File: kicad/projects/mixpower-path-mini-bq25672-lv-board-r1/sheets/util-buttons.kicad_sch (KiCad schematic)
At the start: 15 parts, among them SW1 TS-A002, SW2 TS-A002, SW3 TS-A002, U11 RT9829GQW, U9 RT9829GQW

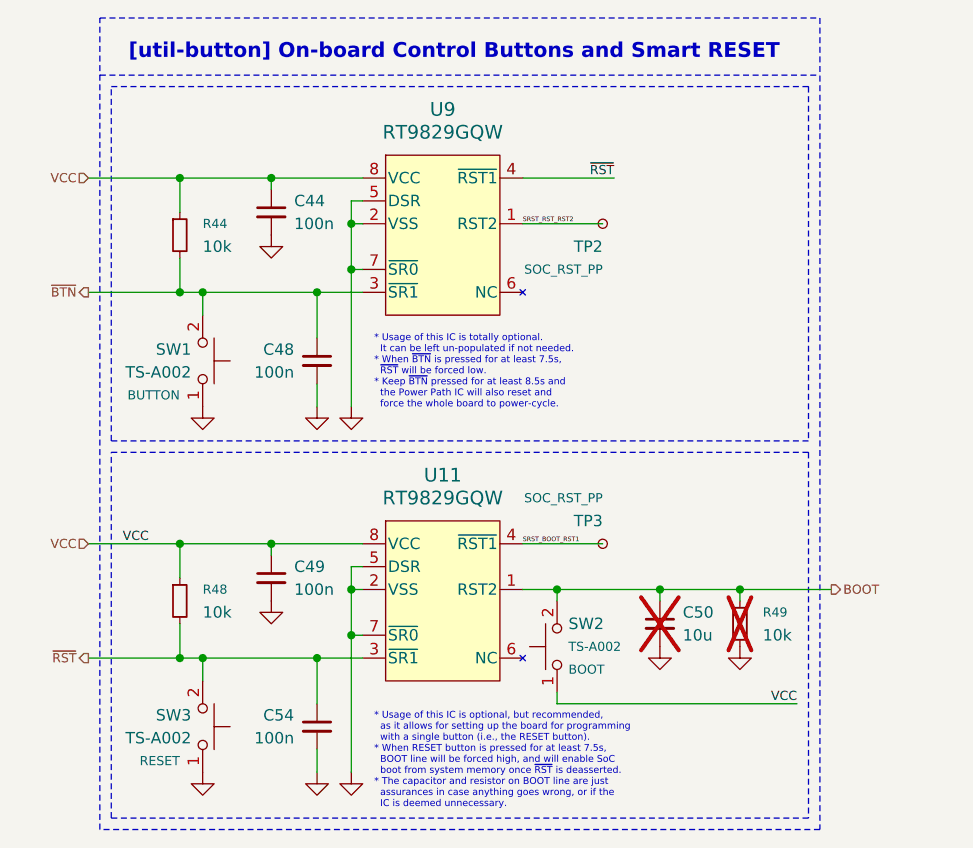
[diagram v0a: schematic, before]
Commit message: feat: small changes in schematics, some PCB routing
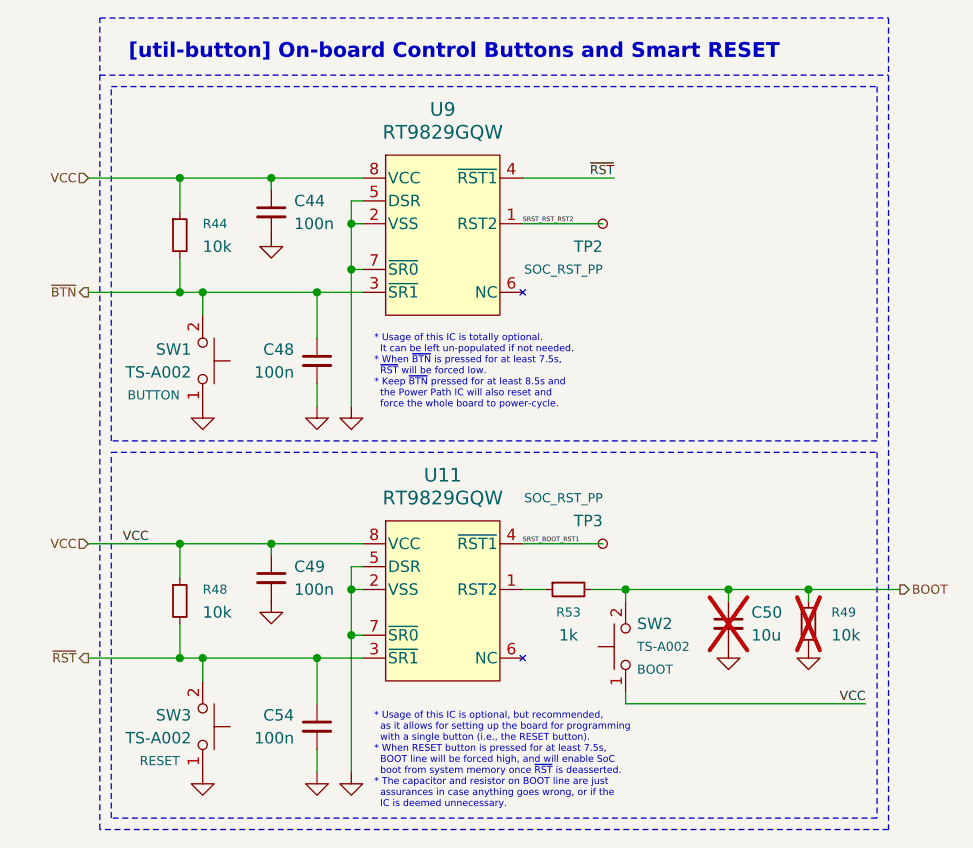
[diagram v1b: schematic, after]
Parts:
- added R53: 1k, Resistor_SMD:R_0402_1005Metric, symbol Device:R_Small
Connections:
- net BOOT: now also R53.2; no longer U11.1 (RST2)
- new net: R53.1, U11.1 (RST2)
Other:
- moved on the sheet: C50, R49, SW2
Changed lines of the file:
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@@
 	(rectangle
 		(start 68.58 24.13)
-		(end 146.05 63.5)
+		(end 153.67 63.5)
 		(stroke
 			(width 0)
@@
 	(rectangle
 		(start 67.31 16.51)
-		(end 147.32 106.68)
+		(end 154.94 106.68)
 		(stroke
 			(width 0)
@@
 	(rectangle
 		(start 68.58 64.77)
-		(end 146.05 105.41)
+		(end 153.67 105.41)
 		(stroke
 			(width 0)
@@
 	)
 	(junction
-		(at 129.54 80.01)
+		(at 137.16 80.01)
 		(diameter 0)
 		(color 0 0 0 0)
@@
 	)
 	(junction
-		(at 138.43 80.01)
+		(at 146.05 80.01)
 		(diameter 0)
 		(color 0 0 0 0)
@@
 	)
 	(junction
-		(at 118.11 80.01)
+		(at 125.73 80.01)
 		(diameter 0)
 		(color 0 0 0 0)
@@
 	(wire
 		(pts
-			(xy 129.54 80.01) (xy 138.43 80.01)
+			(xy 137.16 80.01) (xy 146.05 80.01)
 		)
 		(stroke
@@
 	(wire
 		(pts
-			(xy 118.11 80.01) (xy 118.11 81.28)
+			(xy 125.73 80.01) (xy 125.73 81.28)
 		)
 		(stroke
@@
 	(wire
 		(pts
+			(xy 121.92 80.01) (xy 125.73 80.01)
+		)
+		(stroke
+			(width 0)
+			(type default)
+		)
+	)
+	(wire
+		(pts
 			(xy 95.25 77.47) (xy 95.25 80.01)
 		)
@@
 	(polyline
 		(pts
-			(xy 67.31 22.86) (xy 147.32 22.86)
+			(xy 67.31 22.86) (xy 154.94 22.86)
 		)
 		(stroke
@@
 	(wire
 		(pts
-			(xy 129.54 80.01) (xy 129.54 81.28)
+			(xy 137.16 80.01) (xy 137.16 81.28)
 		)
 		(stroke
@@
 	(wire
 		(pts
-			(xy 118.11 92.71) (xy 144.78 92.71)
+			(xy 125.73 92.71) (xy 152.4 92.71)
 		)
 		(stroke
@@
 	(wire
 		(pts
-			(xy 114.3 80.01) (xy 118.11 80.01)
+			(xy 114.3 80.01) (xy 116.84 80.01)
 		)
 		(stroke
@@
 	(wire
 		(pts
-			(xy 138.43 80.01) (xy 148.59 80.01)
+			(xy 146.05 80.01) (xy 156.21 80.01)
 		)
 		(stroke
@@
 	(wire
 		(pts
-			(xy 118.11 91.44) (xy 118.11 92.71)
+			(xy 125.73 91.44) (xy 125.73 92.71)
 		)
 		(stroke
@@
 	(wire
 		(pts
-			(xy 138.43 80.01) (xy 138.43 81.28)
+			(xy 146.05 80.01) (xy 146.05 81.28)
 		)
 		(stroke
@@
 	(wire
 		(pts
-			(xy 118.11 80.01) (xy 129.54 80.01)
+			(xy 125.73 80.01) (xy 137.16 80.01)
 		)
 		(stroke
@@
 	)
 	(label "VCC"
-		(at 144.78 92.71 180)
+		(at 152.4 92.71 180)
 		(effects
 			(font
@@
 	(hierarchical_label "BOOT"
 		(shape output)
-		(at 148.59 80.01 0)
+		(at 156.21 80.01 0)
 		(effects
 			(font
@@
 	(symbol
 		(lib_id "mixlib-electromechanic-switch:TS-A002")
-		(at 118.11 86.36 90)
+		(at 125.73 86.36 90)
 		(unit 1)
 		(exclude_from_sim no)
@@
 		(dnp no)
 		(property "Reference" "SW2"
-			(at 119.38 83.8199 90)
+			(at 127 83.8199 90)
 			(effects
 				(font
@@
 		)
 		(property "Value" "TS-A002"
-			(at 119.38 86.3599 90)
+			(at 127 86.3599 90)
 			(effects
 				(font
@@
 		)
 		(property "Footprint" "mixlib-electromechanic-switch:TS-A002"
-			(at 118.11 86.36 0)
+			(at 125.73 86.36 0)
 			(effects
 				(font
@@
 		)
 		(property "Datasheet" "https://www.hq-dz.com/uploadfile/2024/0305/20240305025619371.pdf"
-			(at 123.444 85.852 0)
+			(at 131.064 85.852 0)
 			(effects
 				(font
@@
 		)
 		(property "Description" "12V 50mA 0.1Ohm MINIATURE SMD SPST BUTTON"
-			(at 124.206 86.868 0)
+			(at 131.826 86.868 0)
 			(effects
 				(font
@@
 		)
 		(property "Role" "BOOT"
-			(at 119.38 88.9 90)
+			(at 127 88.9 90)
 			(effects
 				(font
@@
 	(symbol
 		(lib_id "Device:C_Small")
-		(at 129.54 83.82 0)
+		(at 137.16 83.82 0)
 		(unit 1)
 		(exclude_from_sim no)
@@
 		(dnp yes)
 		(property "Reference" "C50"
-			(at 132.08 82.5562 0)
+			(at 139.7 82.5562 0)
 			(effects
 				(font
@@
 		)
 		(property "Value" "10u"
-			(at 132.08 85.0962 0)
+			(at 139.7 85.0962 0)
 			(effects
 				(font
@@
 		)
 		(property "Footprint" "Capacitor_SMD:C_0402_1005Metric"
-			(at 129.54 83.82 0)
+			(at 137.16 83.82 0)
 			(effects
 				(font
@@
 		)
 		(property "Datasheet" "~"
-			(at 129.54 83.82 0)
+			(at 137.16 83.82 0)
 			(effects
 				(font
@@
 		)
 		(property "Description" "Unpolarized capacitor, small symbol"
-			(at 129.54 83.82 0)
+			(at 137.16 83.82 0)
 			(effects
 				(font
@@
 	(symbol
 		(lib_id "power:GND")
-		(at 129.54 86.36 0)
+		(at 137.16 86.36 0)
 		(unit 1)
 		(exclude_from_sim no)
@@
 		(fields_autoplaced yes)
 		(property "Reference" "#PWR082"
-			(at 129.54 92.71 0)
+			(at 137.16 92.71 0)
 			(effects
 				(font
@@
 		)
 		(property "Value" "GND"
-			(at 129.54 91.44 0)
+			(at 137.16 91.44 0)
 			(effects
 				(font
@@
 		)
 		(property "Footprint" ""
-			(at 129.54 86.36 0)
+			(at 137.16 86.36 0)
 			(effects
 				(font
@@
 		)
 		(property "Datasheet" ""
-			(at 129.54 86.36 0)
+			(at 137.16 86.36 0)
 			(effects
 				(font
@@
 		)
 		(property "Description" "Power symbol creates a global label with name \"GND\" , ground"
-			(at 129.54 86.36 0)
+			(at 137.16 86.36 0)
 			(effects
 				(font
@@
 	(symbol
 		(lib_id "power:GND")
-		(at 138.43 86.36 0)
+		(at 146.05 86.36 0)
 		(unit 1)
 		(exclude_from_sim no)
@@
 		(fields_autoplaced yes)
 		(property "Reference" "#PWR083"
-			(at 138.43 92.71 0)
+			(at 146.05 92.71 0)
 			(effects
 				(font
@@
 		)
 		(property "Value" "GND"
-			(at 138.43 91.44 0)
+			(at 146.05 91.44 0)
 			(effects
 				(font
@@
 		)
 		(property "Footprint" ""
-			(at 138.43 86.36 0)
+			(at 146.05 86.36 0)
 			(effects
 				(font
@@
 		)
 		(property "Datasheet" ""
-			(at 138.43 86.36 0)
+			(at 146.05 86.36 0)
 			(effects
 				(font
@@
 		)
 		(property "Description" "Power symbol creates a global label with name \"GND\" , ground"
-			(at 138.43 86.36 0)
+			(at 146.05 86.36 0)
 			(effects
 				(font
@@
 	)
 	(symbol
+		(lib_id "Device:R_Small")
+		(at 119.38 80.01 90)
+		(mirror x)
+		(unit 1)
+		(exclude_from_sim no)
+		(in_bom yes)
+		(on_board yes)
+		(dnp no)
+		(property "Reference" "R53"
+			(at 119.38 82.55 90)
+			(effects
+				(font
+					(size 1.016 1.016)
+				)
+			)
+		)
+		(property "Value" "1k"
+			(at 119.38 85.09 90)
+			(effects
+				(font
+					(size 1.27 1.27)
+				)
+			)
+		)
+		(property "Footprint" "Resistor_SMD:R_0402_1005Metric"
+			(at 119.38 80.01 0)
+			(effects
+				(font
+					(size 1.27 1.27)
+				)
+				(hide yes)
+			)
+		)
+		(property "Datasheet" "~"
+			(at 119.38 80.01 0)
+			(effects
+				(font
+					(size 1.27 1.27)
+				)
+				(hide yes)
+			)
+		)
+		(property "Description" "Resistor, small symbol"
+			(at 119.38 80.01 0)
+			(effects
+				(font
+					(size 1.27 1.27)
+				)
+				(hide yes)
+			)
+		)
+		(pin "2"
+		)
+		(pin "1"
+		)
+		(instances
+			(project "mixpower-path-mini-bq25672-lv-board-r1"
+				(path "/2e43857b-9bf9-460c-948c-ec2cf8a8d6b4/02edf1bd-e23a-4a4a-8860-4d5790274652"
+					(reference "R53")
+					(unit 1)
+				)
+			)
+		)
+	)
+	(symbol
 		(lib_id "power:GND")
 		(at 91.44 100.33 0)
@@
 	(symbol
 		(lib_id "Device:R_Small")
-		(at 138.43 83.82 0)
+		(at 146.05 83.82 0)
 		(unit 1)
 		(exclude_from_sim no)
@@
 		(fields_autoplaced yes)
 		(property "Reference" "R49"
-			(at 140.97 82.5499 0)
+			(at 148.59 82.5499 0)
 			(effects
 				(font
@@
 		)
 		(property "Value" "10k"
-			(at 140.97 85.0899 0)
+			(at 148.59 85.0899 0)
 			(effects
 				(font
@@
 		)
 		(property "Footprint" "Resistor_SMD:R_0402_1005Metric"
-			(at 138.43 83.82 0)
+			(at 146.05 83.82 0)
 			(effects
 				(font
@@
 		)
 		(property "Datasheet" "~"
-			(at 138.43 83.82 0)
+			(at 146.05 83.82 0)
 			(effects
 				(font
@@
 		)
 		(property "Description" "Resistor, small symbol"
-			(at 138.43 83.82 0)
+			(at 146.05 83.82 0)
 			(effects
 				(font
